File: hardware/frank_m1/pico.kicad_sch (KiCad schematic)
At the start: 2 parts, among them U4 Rasberry Pi Pico

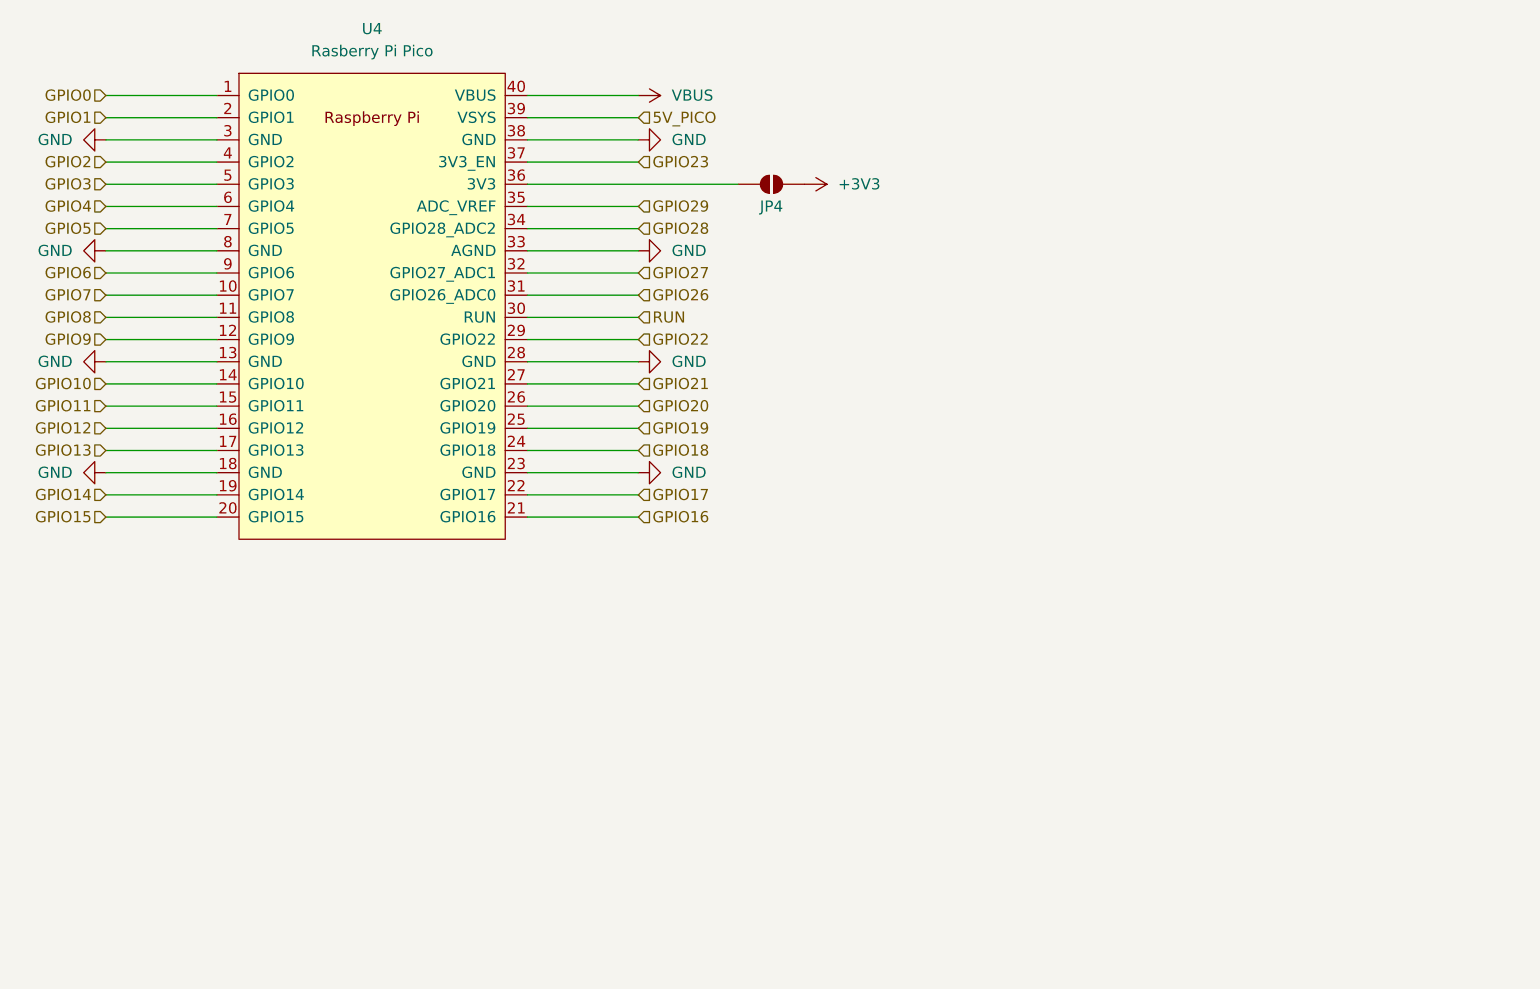
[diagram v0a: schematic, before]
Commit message: Minor updates
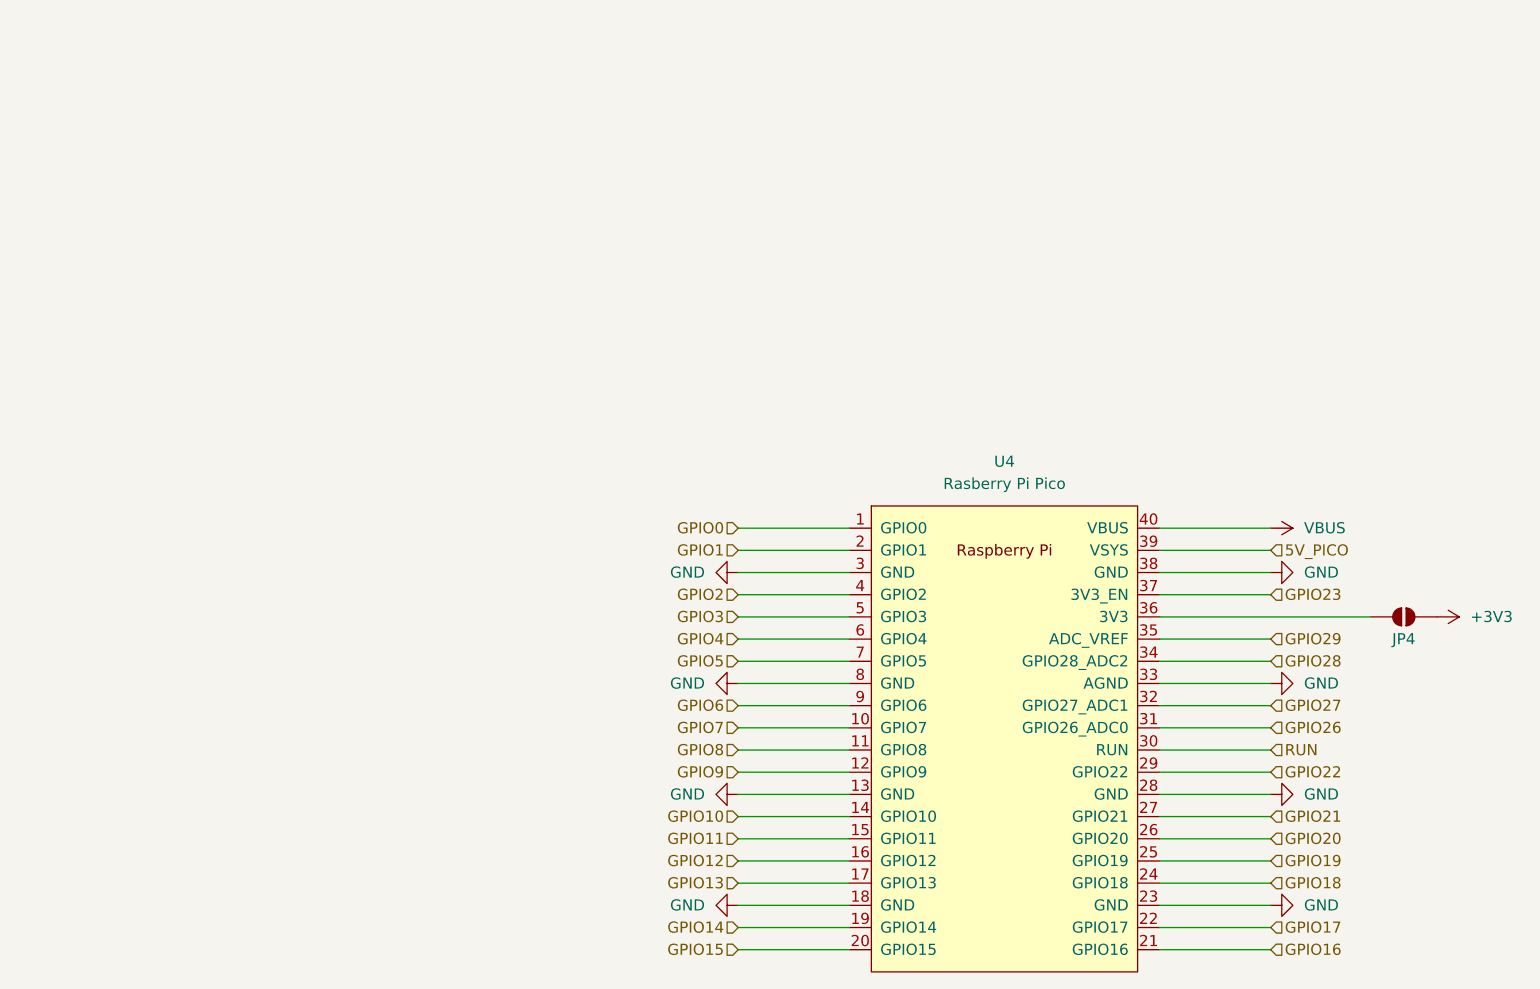
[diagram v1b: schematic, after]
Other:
- moved on the sheet: JP4, U4
